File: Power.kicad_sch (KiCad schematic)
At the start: 38 parts, among them U2 SCT2610, U4 SCT2420

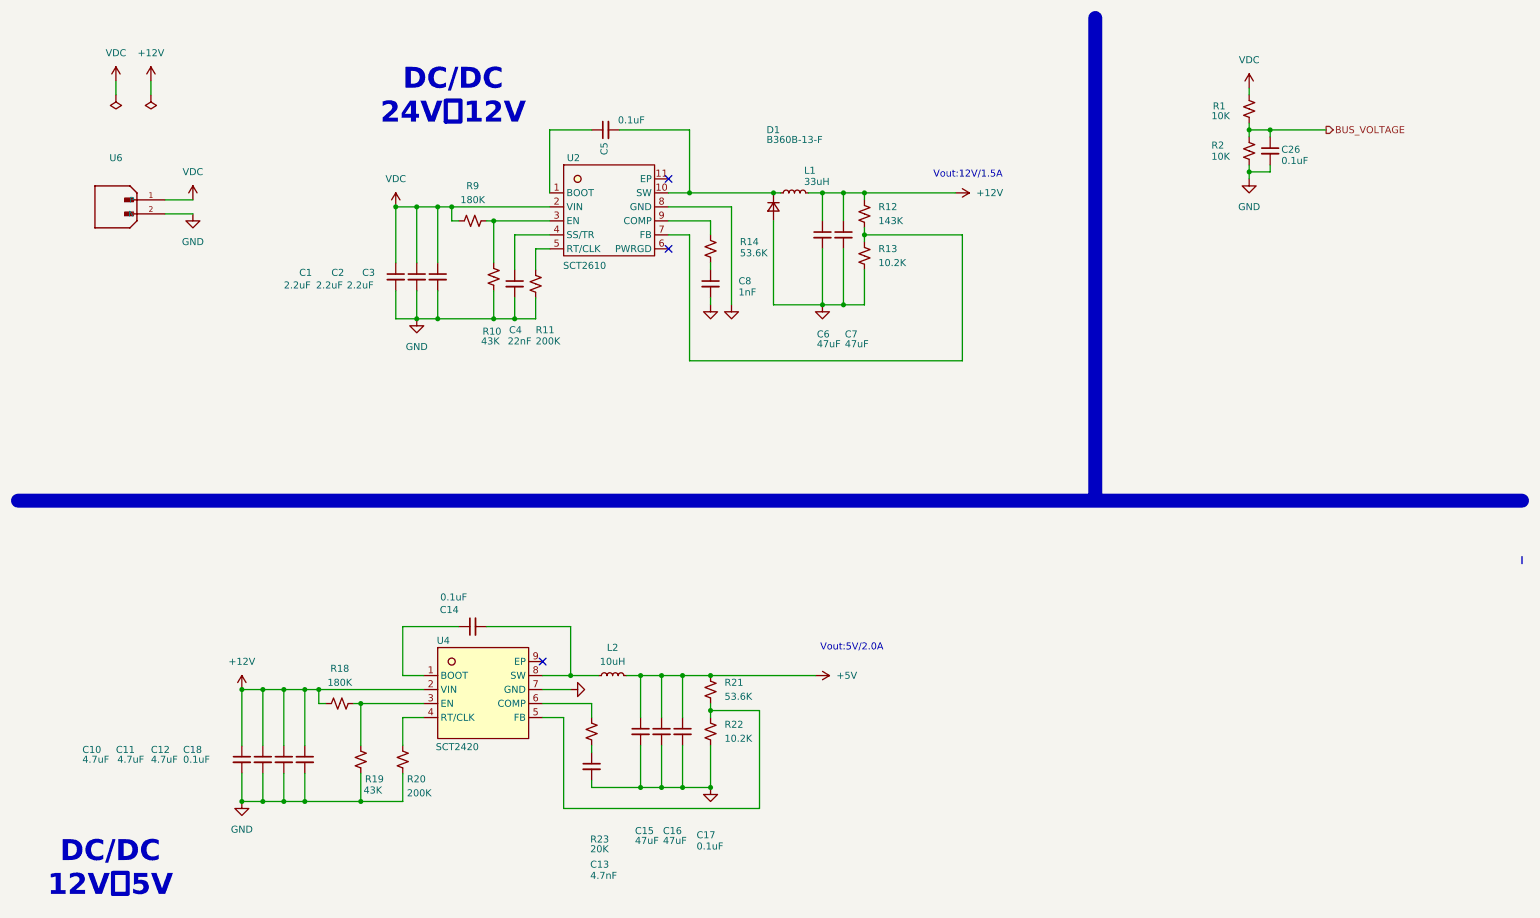
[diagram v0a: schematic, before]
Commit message: 优化原理图
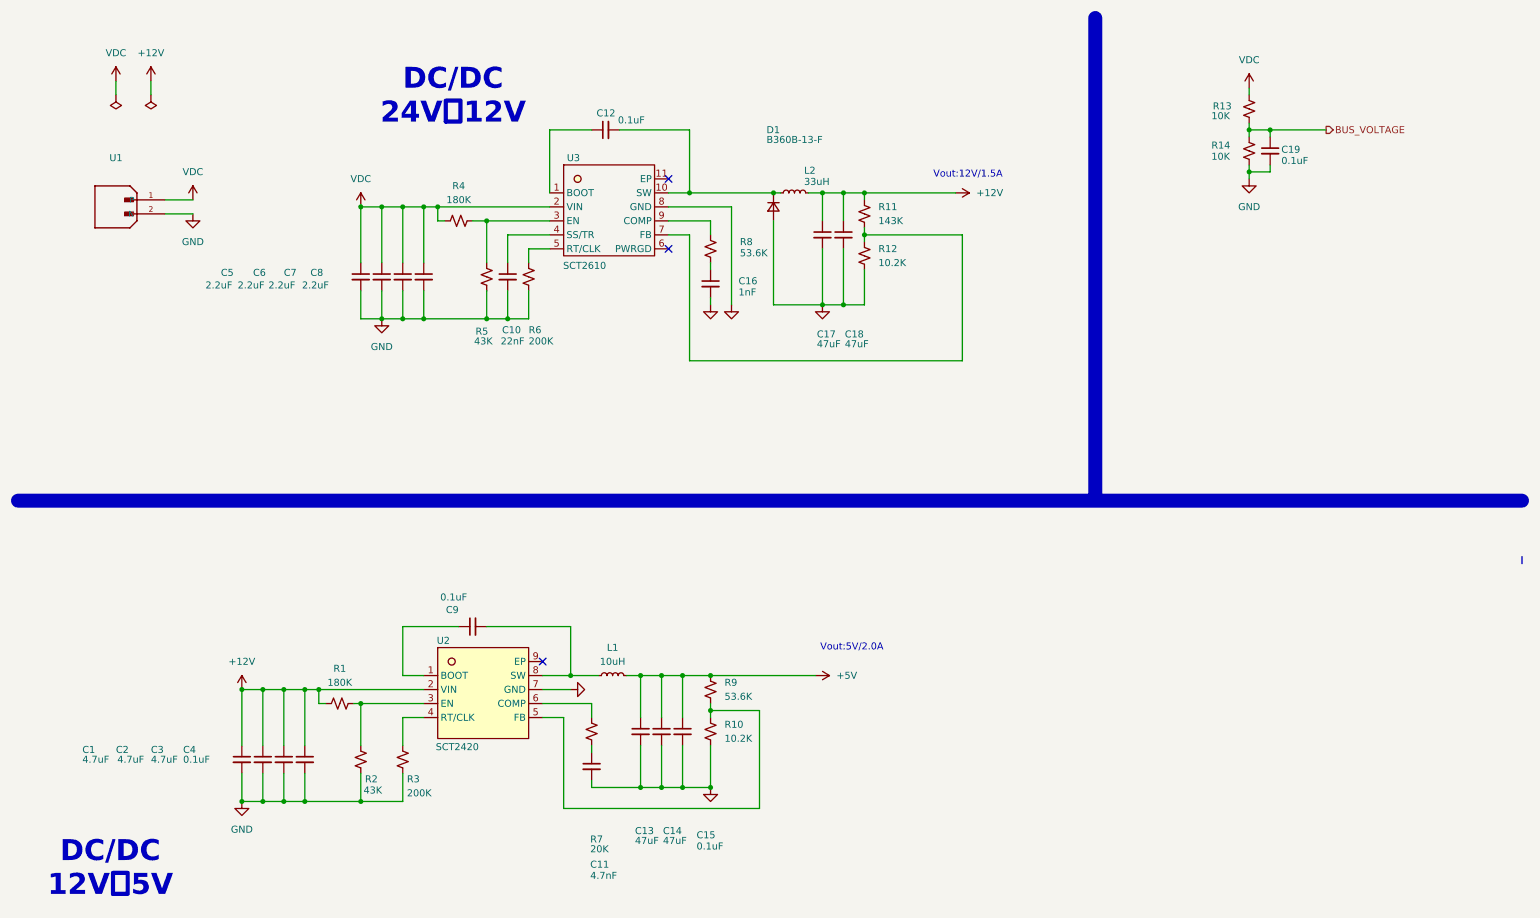
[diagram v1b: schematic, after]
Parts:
- added C8: 2.2uF, Capacitor_SMD:C_0603_1608Metric, symbol Device:C_Small
- renumbered C10 to C1, C4 to C10, C13 to C11, C5 to C12, C15 to C13, C16 to C14, C17 to C15, C8 to C16, C6 to C17, C7 to C18, C26 to C19, C11 to C2, C12 to C3, C18 to C4, C1 to C5, C2 to C6, C3 to C7, C14 to C9, L2 to L1, L1 to L2, R18 to R1, R22 to R10, R12 to R11, R13 to R12, R1 to R13, R2 to R14, R19 to R2, R20 to R3, R9 to R4, R10 to R5, R11 to R6, R23 to R7, R14 to R8, R21 to R9, U6 to U1, U4 to U2, U2 to U3
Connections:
- net GND: now also C8.2
- net VDC: now also C8.1
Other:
- moved on the sheet: C10, C5, C6, C7, R4, R5, R6
